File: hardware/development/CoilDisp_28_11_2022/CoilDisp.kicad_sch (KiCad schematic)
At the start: 119 parts, among them J1 E_ANT, J10 E2154CS0C1, J2 E_ANT, J3 UFL, J4 HV OUT, J6 3.3 OUT, J8 GND, J9 SWD, Q1 SSM6N36TU, Q3 BC846W, Q4 PMZB390UNE, SW1 EVQ-P2202M, SW2 EVQ-P2202M, SW3 EVQ-P2202M, U1 TPS62171DSG, U2 STM32L432KCUx, Y1 FC2012AN

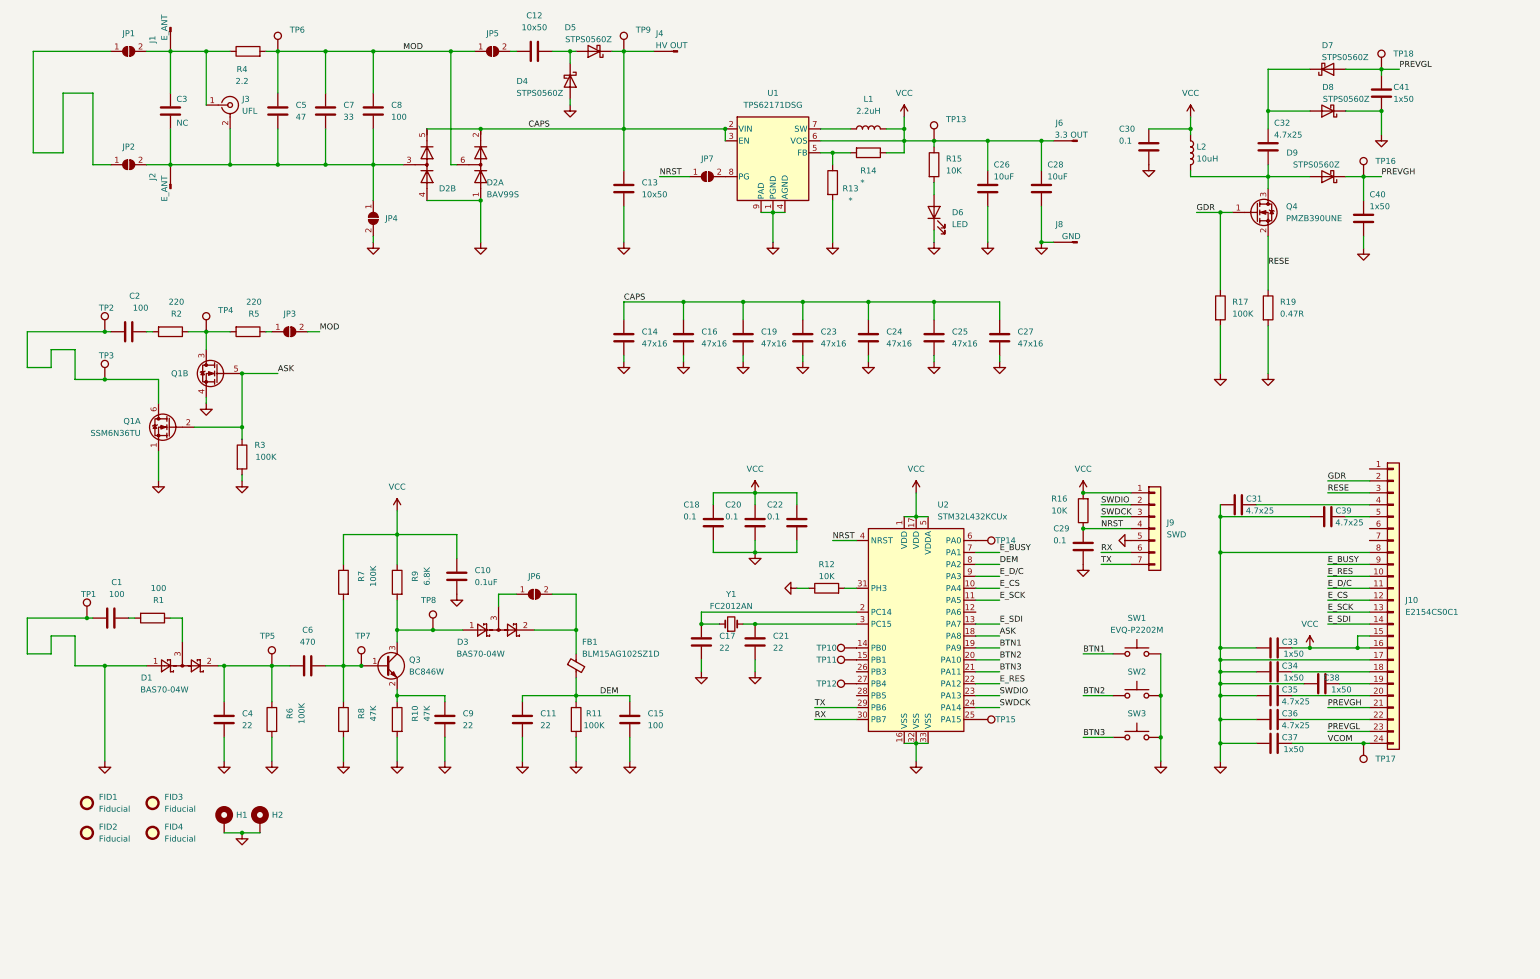
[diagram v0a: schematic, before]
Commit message: docs: document schematics
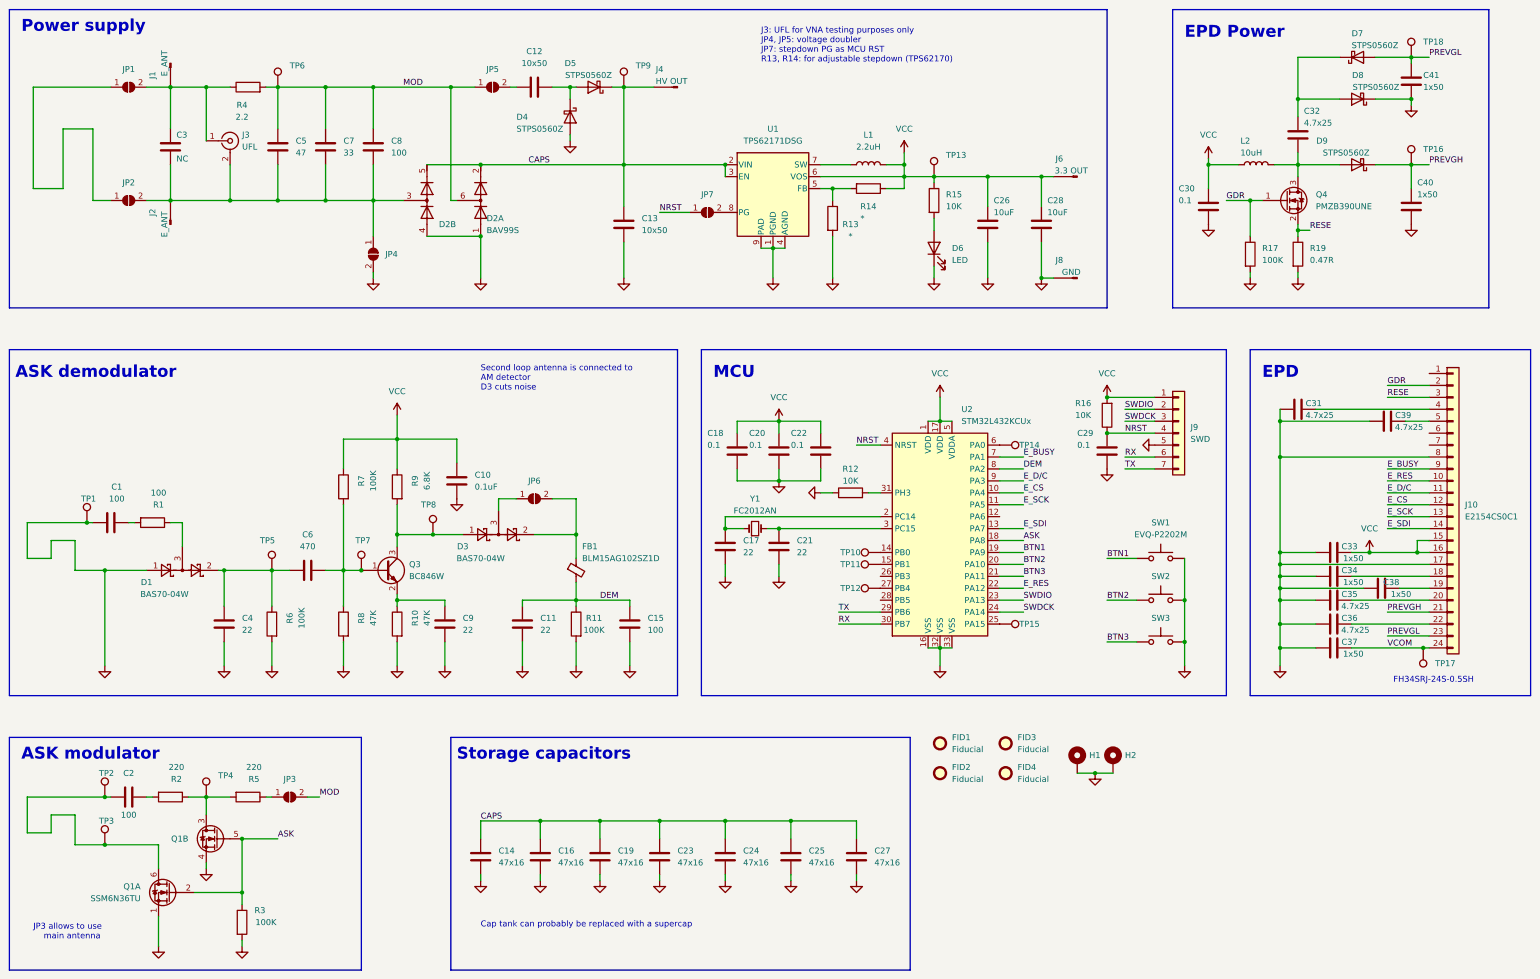
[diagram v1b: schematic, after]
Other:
- note added: "ASK demodulator"
- note added: "ASK modulator"
- note added: "Cap tank can probably be replaced with a supercap"
- note added: "EPD"
- note added: "EPD Power"
- note added: "FH34SRJ-24S-0.5SH"
- note added: "J3: UFL for VNA testing purposes only JP4, JP5: voltage doubler JP7: stepdown PG as MCU RST R13, R14: for adjustable stepdown (TPS62170)"
- note added: "JP3 allows to use main antenna"
- note added: "MCU"
- note added: "Power supply"
- note added: "Second loop antenna is connected to AM detector D3 cuts noise"
- note added: "Storage capacitors"
- moved on the sheet: C1, C10, C11, C12, C13, C14, C15, C16, C17, C18, C19, C2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
